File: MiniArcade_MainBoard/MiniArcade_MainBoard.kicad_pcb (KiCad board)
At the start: 2 copper layers, 60 x 55 mm, 31 parts, among them J1 62701021721, J2 Conn_01x05_Pin, J3 Conn_01x06_Pin, J4 F3311A7H121026E200, SW1 EVPAA, U1 ATSAMD21J18A-A, U2 LM321

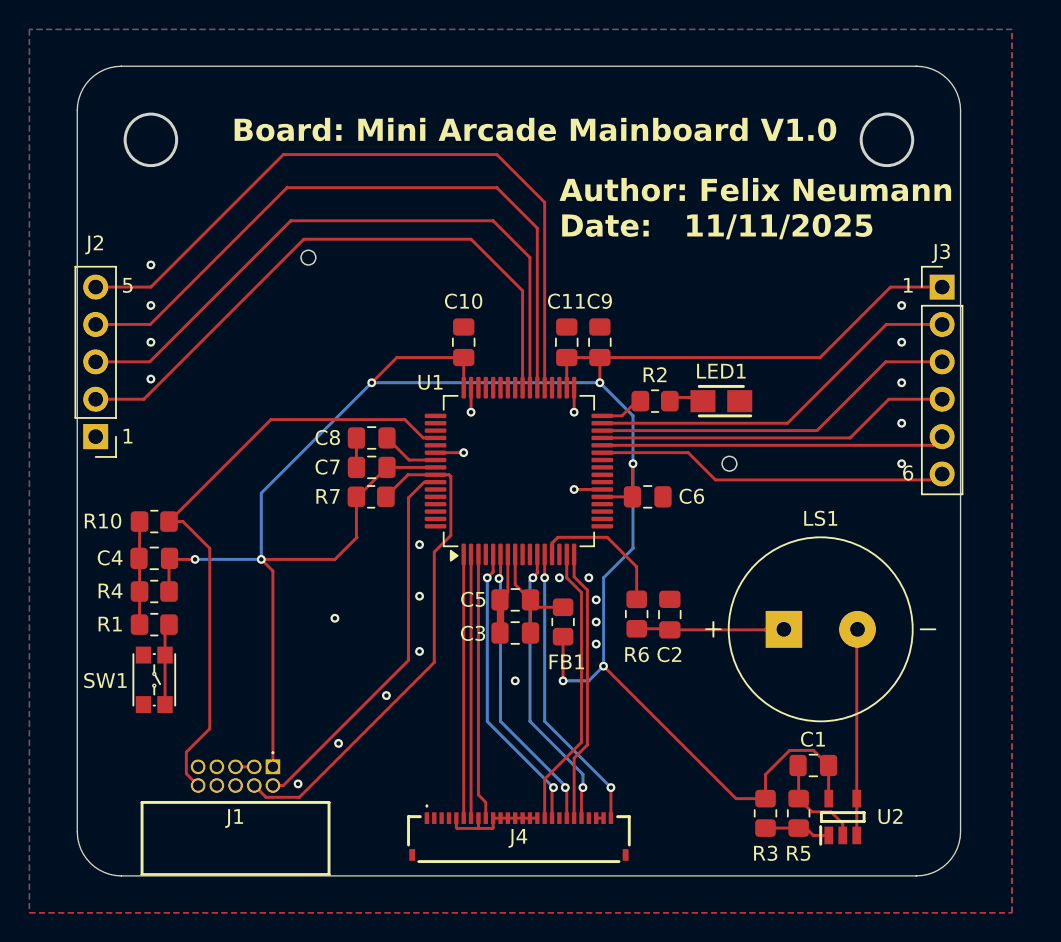
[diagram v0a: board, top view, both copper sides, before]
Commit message: 19 11 2025
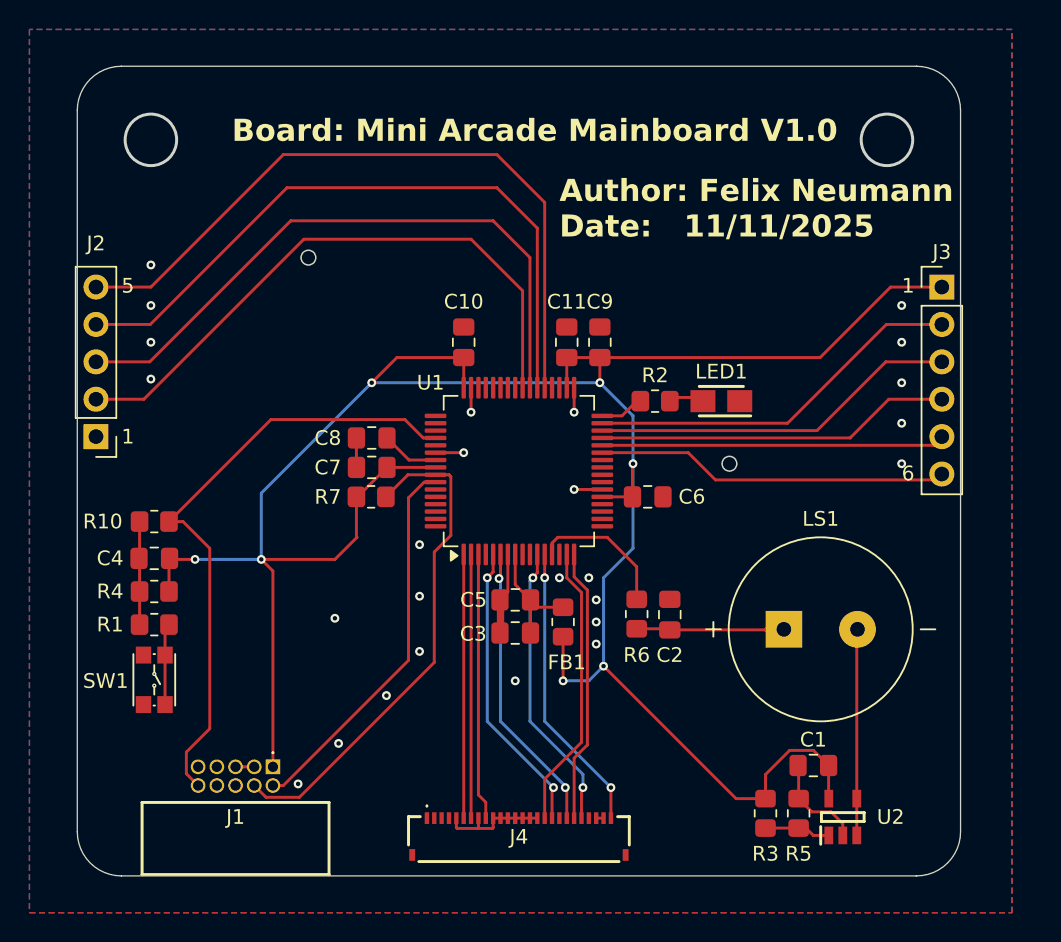
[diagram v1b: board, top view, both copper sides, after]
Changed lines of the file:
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@@
 	(footprint "Connector_PinHeader_2.54mm:PinHeader_1x06_P2.54mm_Vertical"
 		(layer "F.Cu")
-		(at 168.75 105)
+		(at 168.73 105)
 		(descr "Through hole straight pin header, 1x06, 2.54mm pitch, single row")
 		(tags "Through hole pin header THT 1x06 2.54mm single row")
@@
 	(footprint "Connector_PinHeader_2.54mm:PinHeader_1x05_P2.54mm_Vertical"
 		(layer "F.Cu")
-		(at 111.25 115.16 180)
+		(at 111.27 115.16 180)
 		(descr "Through hole straight pin header, 1x05, 2.54mm pitch, single row")
 		(tags "Through hole pin header THT 1x05 2.54mm single row")
@@
 		(hatch edge 0.5)
 		(connect_pads
-			(clearance 0.5)
+			(clearance 0.3)
 		)
 		(min_thickness 0.25)
